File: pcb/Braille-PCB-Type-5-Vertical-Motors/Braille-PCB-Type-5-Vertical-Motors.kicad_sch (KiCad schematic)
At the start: 40 parts, among them J101 Conn_01x02, J102 Screw_Terminal_01x02, J103 Screw_Terminal_01x02, J104 Screw_Terminal_01x02, J105 Conn_01x05, J106 Conn_01x05, J107 Conn_01x08, J108 Conn_01x05, J109 Conn_01x05, SW101 SW_Push, SW102 SW_Push, U101 RP2040-Zero, U102 AMS1117-3.3, U103 INA219AxD

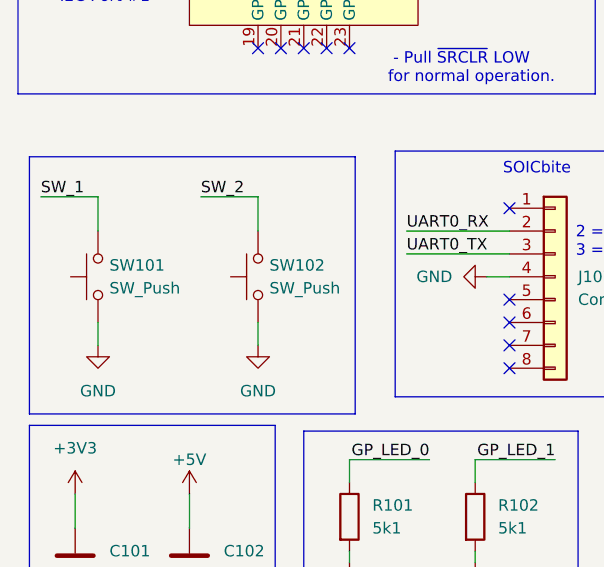
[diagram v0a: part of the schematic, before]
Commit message: chore: bump KiCAD to v9, maybe other minor changes
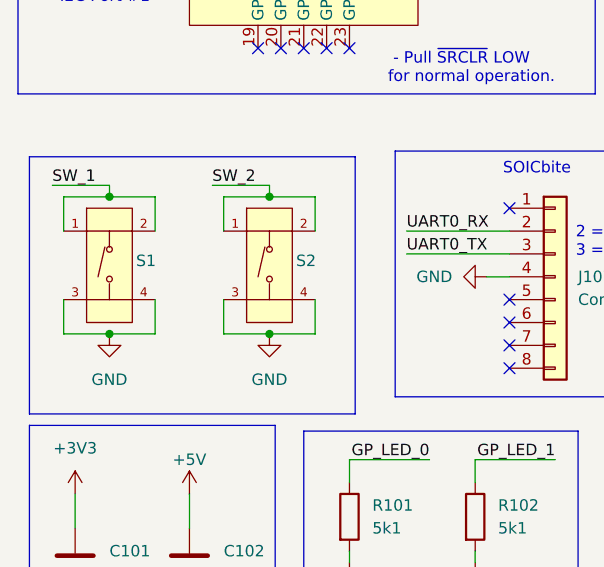
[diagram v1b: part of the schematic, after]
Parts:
- removed SW101, SW102: SW_Push, 00-project-footprints:PushButtonSMD_2.93x3.9, symbol Switch:SW_Push
- added S1, S2: Tactile Button, 160gf, PCM_JLCPCB:SW-SMD_4P-L5.1-W5.1-P3.70-LS6.5-TL-2, symbol PCM_JLCPCB-Connectors_Buttons:Tactile Button, 160gf
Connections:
- net GND: now also S1.3 (C), S1.4 (D), S2.3 (C), S2.4 (D)
- net SW_1: now also S1.1 (A), S1.2 (B)
- net SW_2: now also S2.1 (A), S2.2 (B)
